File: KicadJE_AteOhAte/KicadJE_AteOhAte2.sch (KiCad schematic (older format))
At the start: 110 parts, among them J201 In_Accent, J202 In Gate, J203 Out Tom, P201 Doepfer_Power_10pin, Q201 MMBT2222A, Q202 MMBT2222A, Q203 MMBT2222A, Q204 MMBT2222A, Q205 MMBT2907A, Q206 MMBT2222A, Q207 MMBT2222A, SW201 Con/Tom, U201 TL072, U202 TL072, U203 TL072

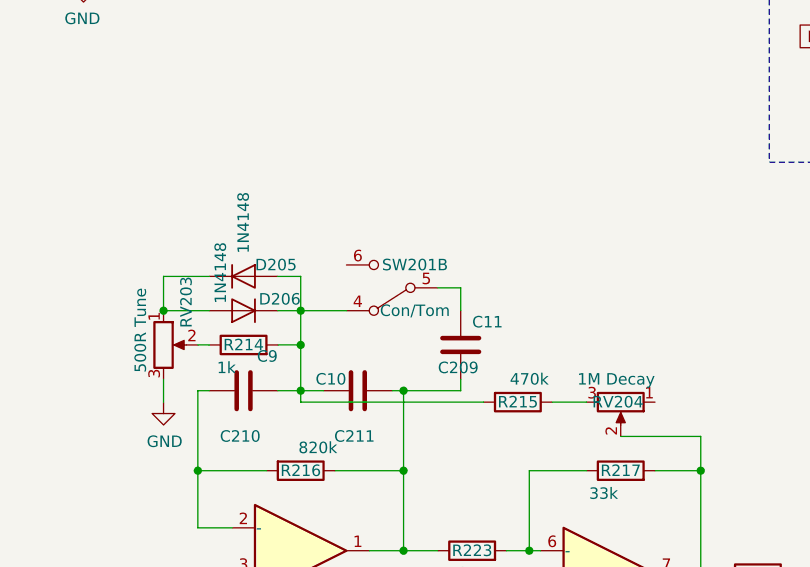
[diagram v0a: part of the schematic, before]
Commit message: pcb
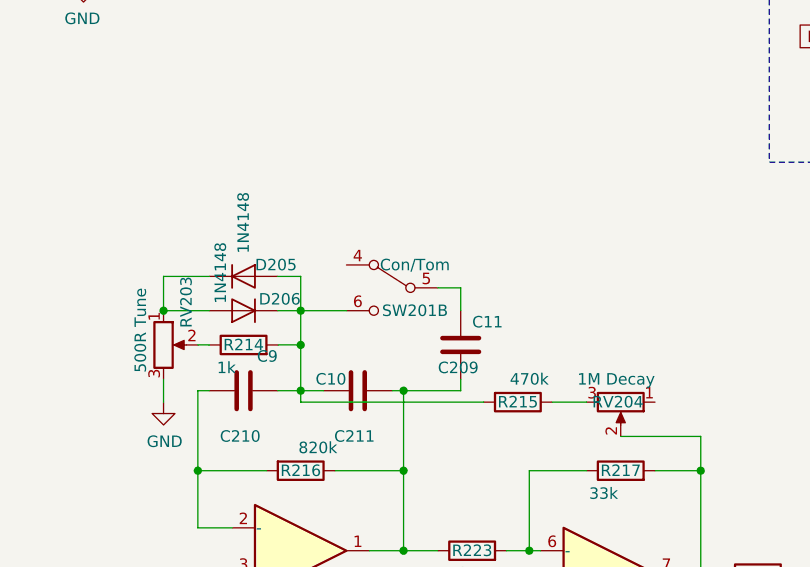
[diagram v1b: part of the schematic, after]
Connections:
- net at C210.2, C211.1, D205.2 (A)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: now also SW201.6 (C); no longer SW201.4 (A)
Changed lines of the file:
@@
 F 3 "~" H 5550 3850 50  0001 C CNN
 	2    5550 3850
-	-1   0    0    1
+	-1   0    0    -1
 $EndComp
 $Comp
